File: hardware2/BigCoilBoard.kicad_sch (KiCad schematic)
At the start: 140 parts, among them J1 Conn_01x02, J10 PFC_OUT, J11 THERM2_IN, J12 THERM3_IN, J13 THERM4_IN, J14 THERM5_IN, J16 Conn_ARM_JTAG_SWD_10, J17 Conn_01x04, J18 Conn_01x04, J19 Conn_01x04, J2 Conn_01x02, J20 Screw_Terminal_01x01, J21 Screw_Terminal_01x01, J22 Screw_Terminal_01x01, J23 Screw_Terminal_01x01, J24 Conn_01x04, J3 Conn_01x03_Pin, J5 THERM1_IN, J6 Conn_01x03_Pin, J7 Conn_01x04, J8 CONTACTOR_1, J9 CONTACTOR_2, K1 G5NB-1A-DC24, K2 G5NB-1A-DC24, Q1 T2N7002AK, Q2 T2N7002AK, Q3 T2N7002AK, Q4 T2N7002AK, Q5 T2N7002AK, Q6 T2N7002AK, Q7 T2N7002AK, U1 STM32G474CBTx, U10 IF-D95, U11 IF-E96E, U12 LD1117S33TR_SOT223, U13 TC7662Bx0A, U14 L7812, U2 MCP6477-E/SN, U3 CSTNE8M00G550000R0, U6 MGJ2D241709SC, U7 STGAP2SM, U8 SN74LV1T34DBV, U9 IF-D95

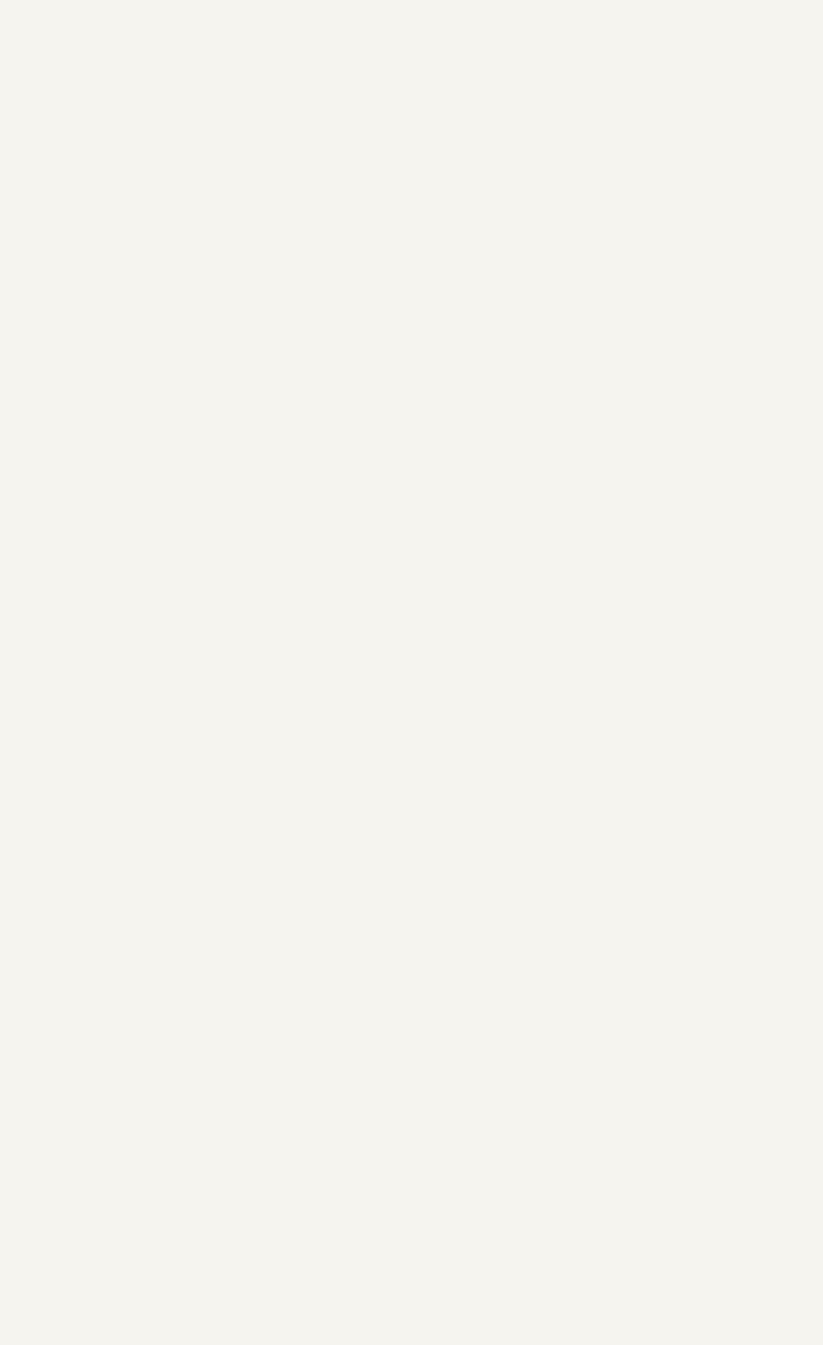
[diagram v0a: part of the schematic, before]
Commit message: idk
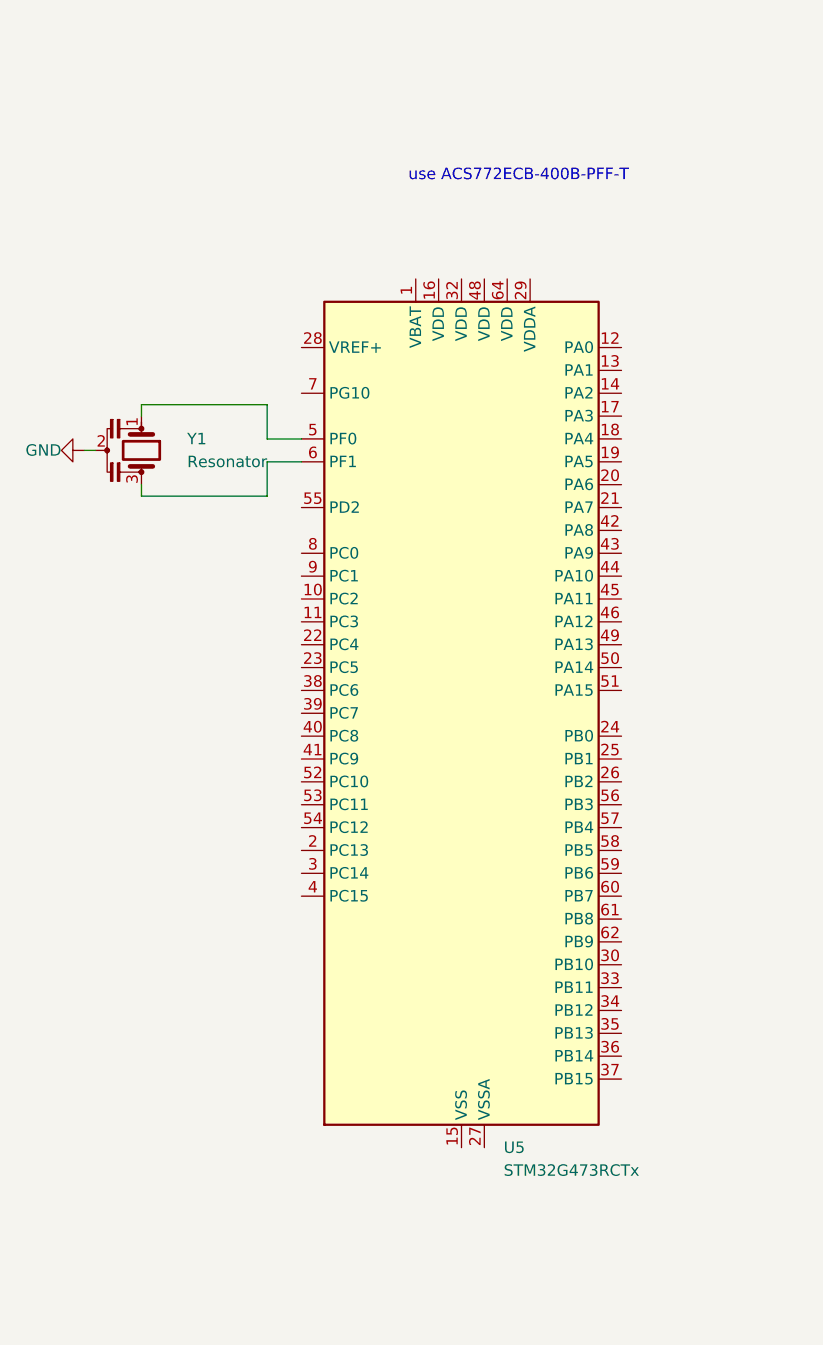
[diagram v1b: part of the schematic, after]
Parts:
- added U5: STM32G473RCTx, Package_QFP:LQFP-64_10x10mm_P0.5mm, symbol MCU_ST_STM32G4:STM32G473RCTx
- added Y1: Resonator, Crystal:Resonator_SMD_Murata_CSTxExxV-3Pin_3.0x1.1mm, symbol Device:Resonator
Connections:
- net GND: now also Y1.2
- new net: U5.15 (VSS), U5.31 (VSS), U5.47 (VSS), U5.63 (VSS)
- new net: U5.5 (PF0), Y1.1
- new net: U5.6 (PF1), Y1.3
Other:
- note added: "use ACS772ECB-400B-PFF-T"
